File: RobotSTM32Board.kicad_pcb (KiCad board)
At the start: 2 copper layers, 70.7 x 88.6 mm, 91 parts, among them IC1 TB6612FNG, IC2 TB6612FNG, J1 MotorA, J10 Qwiik1, J11 Qwiik2, J12 Qwiik3, J13 Qwiik4, J14 Qwiik5, J15 39-30-0040, J15 DCIn, J16 UJC-H-G-SMT-2-P6-TR, J17 BatteryOutputs, J18 BatteryInputs, J2 MotorB, J3 MotorC, J4 MotorD, J5 EncoderA, J6 EncoderB, J7 EncoderC, J8 EncoderD, J9 ESTOP, Q1 NPN, Q2 NMOS_Substrate, Q3 NMOS_Substrate, U1 NUCLEO-F411RE, U3 TPS564252DRLR, U4 TPS51386RJNR, U5 LM27403SQ/NOPB

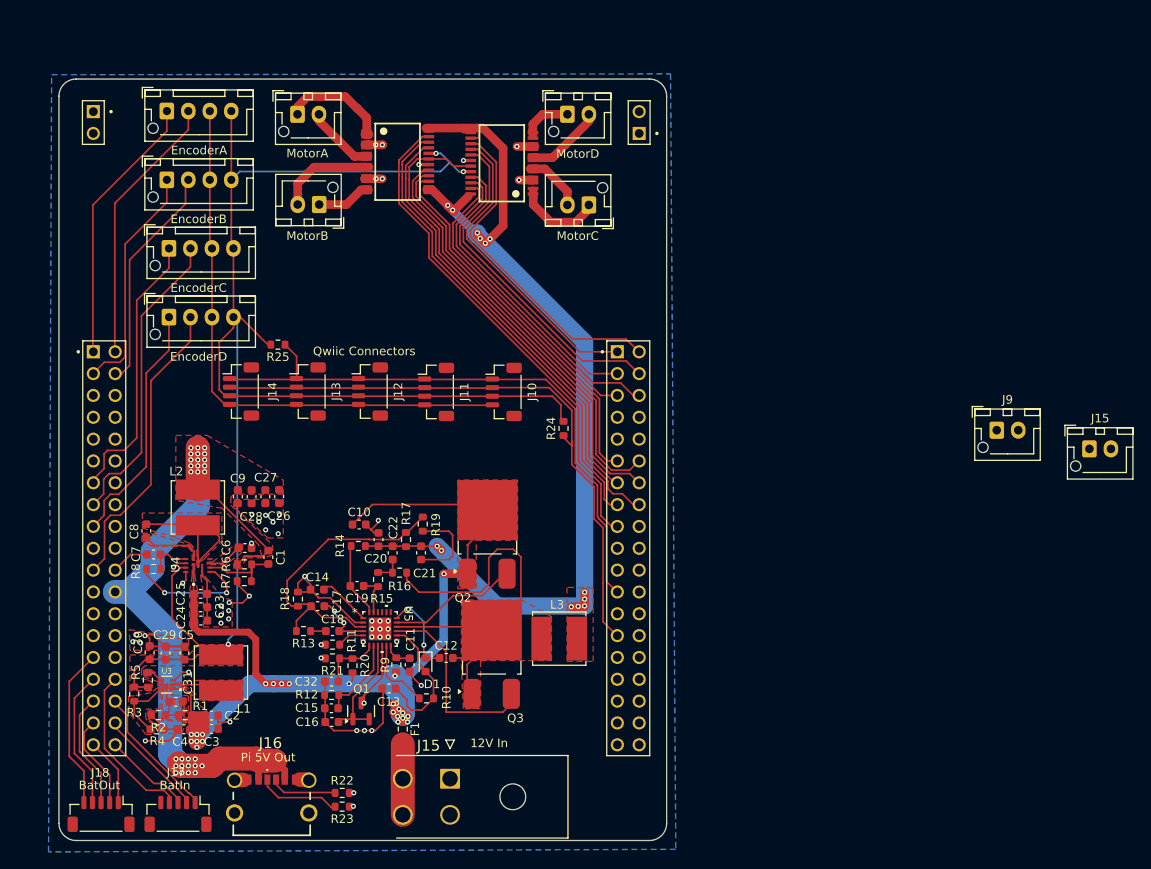
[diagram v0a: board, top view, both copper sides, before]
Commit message: commit of the finished thing before i tidy it up for the report
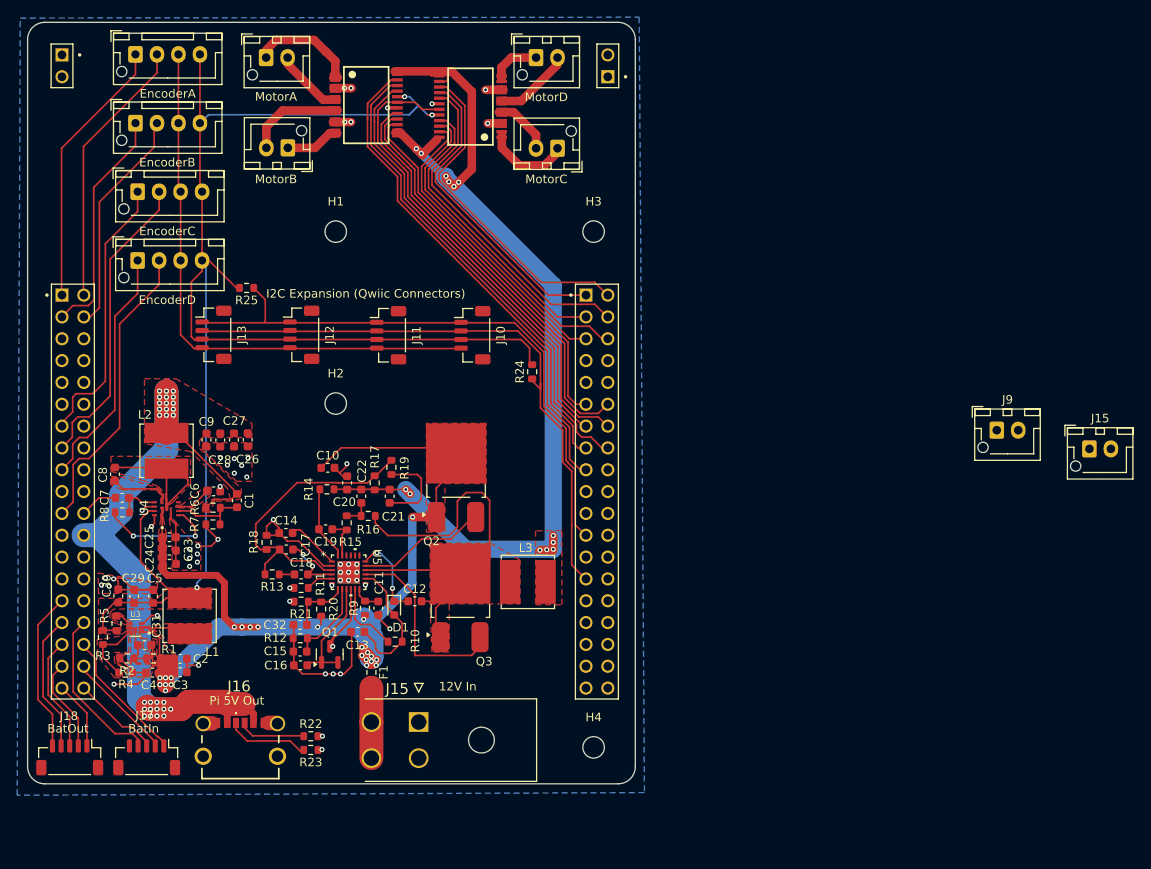
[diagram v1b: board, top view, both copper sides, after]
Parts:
- removed J14: Qwiik5, Connector_JST:JST_SH_BM04B-SRSS-TB_1x04-1MP_P1.00mm_Vertical
- added H1: MountingHole, MountingHole:MountingHole_2.5mm, F.Cu at (140.0, 70.0)
- added H2: MountingHole, MountingHole:MountingHole_2.5mm, F.Cu at (140.0, 90.0)
- added H3: MountingHole, MountingHole:MountingHole_2.5mm, F.Cu at (170.0, 70.0)
- added H4: MountingHole, MountingHole:MountingHole_2.5mm, F.Cu at (170.0, 130.0)
- moved J13 12.8 mm to (125.8, 82.0)
- moved J12 10.3 mm to (136.0, 82.0)
- moved J11 8.63 mm to (146.1, 82.1)
- moved ? 7.54 mm to (141.5, 109.6)
- moved C1 7.54 mm to (128.5, 101.3)
- moved C10 7.54 mm to (139.1, 97.5)
- moved C11 7.54 mm to (145.0, 113.8)
- moved C12 7.54 mm to (149.2, 113.0)
- moved C14 7.54 mm to (134.2, 105.1)
- moved C15 7.54 mm to (135.9, 118.9)
- moved C16 7.54 mm to (135.9, 120.5)
- moved C17 7.54 mm to (134.3, 107.0)
- moved C18 7.54 mm to (136.0, 109.9)
- moved C19 7.54 mm to (138.8, 104.6)
- moved C20 7.54 mm to (143.0, 100.8)
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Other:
- board text added: "I2C Expansion (Qwiic Connectors)"
- board text removed: "Qwiic Connectors"
